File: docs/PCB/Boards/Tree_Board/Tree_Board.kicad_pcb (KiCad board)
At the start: 2 copper layers, 160 x 158 mm, 116 parts, among them Q1 AO3418, Q2 AO3418, SW1 Tact Switch 6x6mm / 13mm, U3 ATtiny85-20S

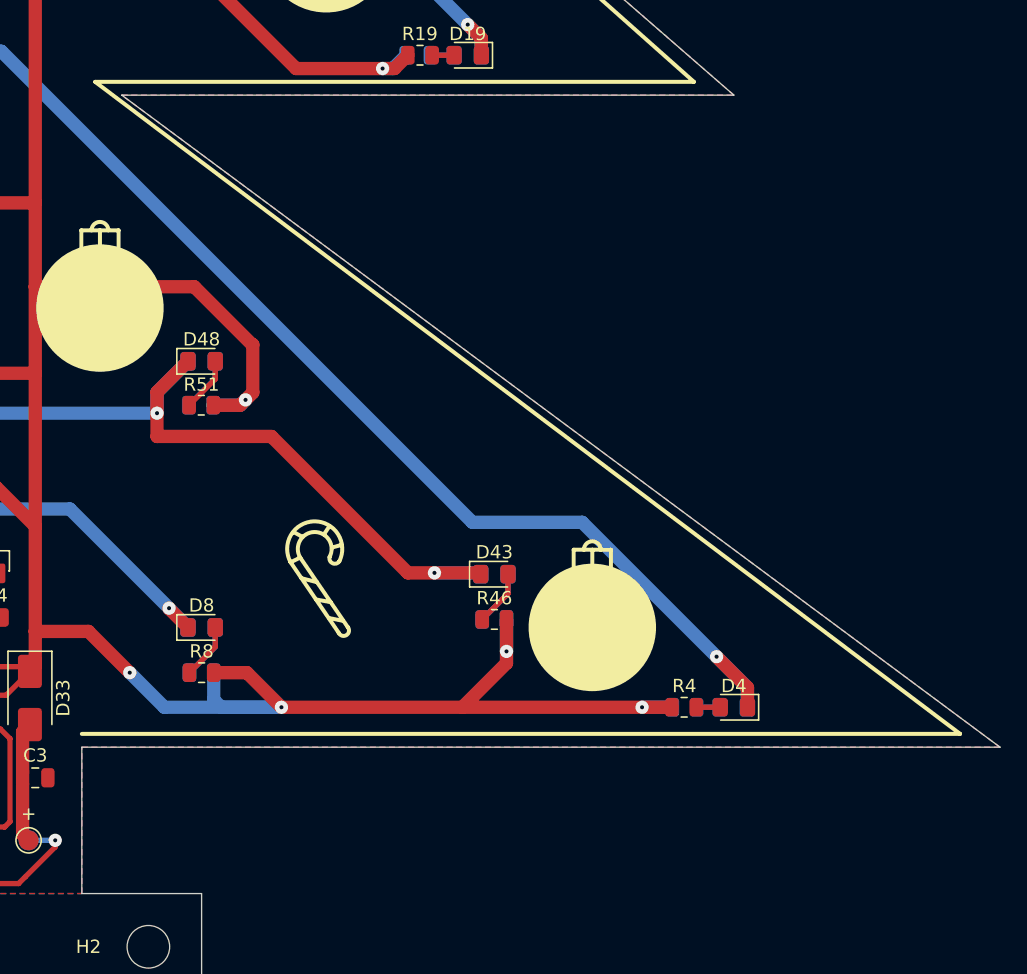
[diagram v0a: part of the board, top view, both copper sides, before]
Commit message: Boards modified.
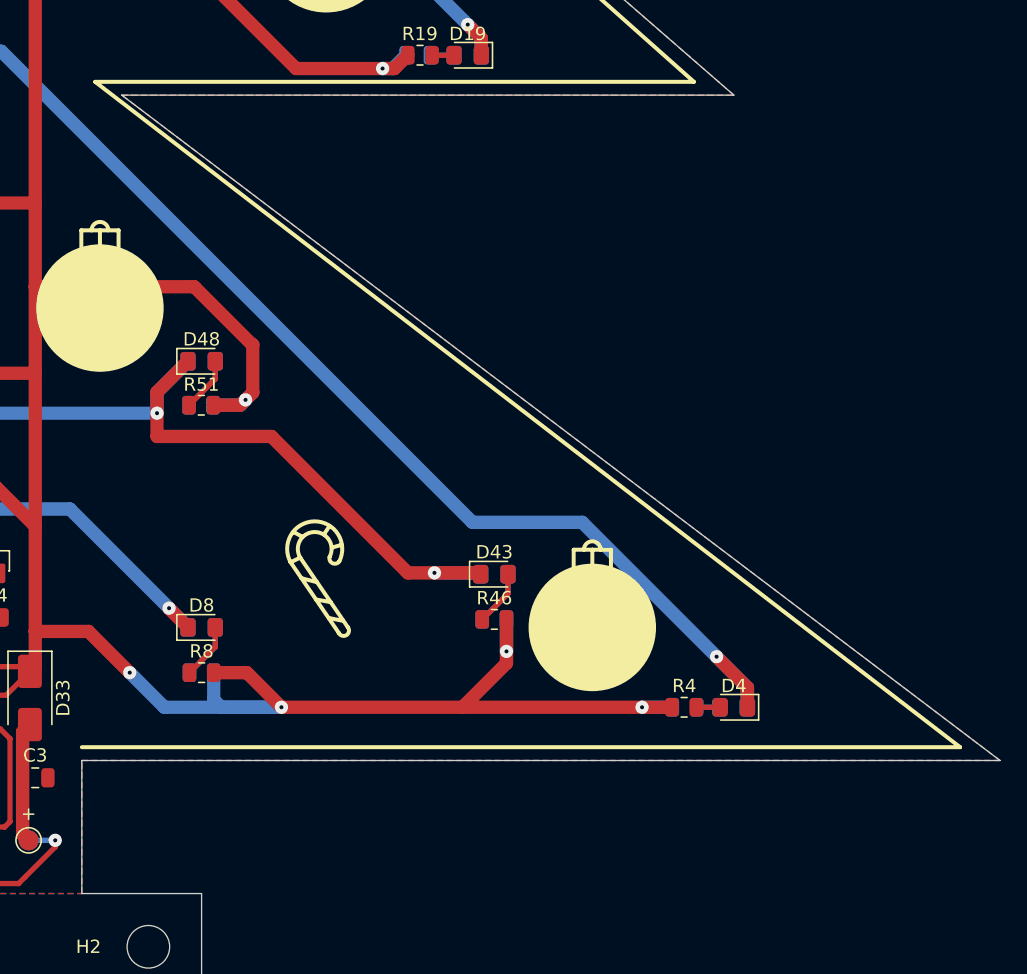
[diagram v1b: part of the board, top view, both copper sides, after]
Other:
- outline, holes or cut-outs redrawn
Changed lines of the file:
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@@
 	(title_block
 		(title "Tree_Board")
-		(date "2025-11-16")
-		(rev "1.0")
+		(date "2025-12-07")
+		(rev "1.1")
 		(company "PKl")
+		(comment 1 "Poprawiony wygląd drzewa.")
 	)
 	(layers
@@
 	)
 	(gr_line
-		(start 197 158)
-		(end 131 158)
+		(start 197 159)
+		(end 131 159)
 		(stroke
 			(width 0.3)
@@
 	(gr_line
 		(start 132 109)
-		(end 197 158)
+		(end 197 159)
 		(stroke
 			(width 0.3)
@@
 	(gr_line
 		(start 132 109)
-		(end 197 158)
+		(end 197 159)
 		(stroke
 			(width 0.3)
@@
 	)
 	(gr_line
-		(start 131 158)
-		(end 197 158)
+		(start 131 159)
+		(end 197 159)
 		(stroke
 			(width 0.3)
@@
 	)
 	(gr_line
-		(start 200 159)
-		(end 131 159)
-		(stroke
-			(width 0.05)
-			(type default)
-		)
-		(layer "Edge.Cuts")
-	)
-	(gr_line
 		(start 131 40)
 		(end 160 70)
@@
 	)
 	(gr_line
-		(start 134 110)
-		(end 200 159)
-		(stroke
-			(width 0.05)
-			(type default)
-		)
-		(layer "Edge.Cuts")
-	)
-	(gr_line
 		(start 40 160)
 		(end 109 160)
@@
 	(gr_line
 		(start 131 170)
-		(end 131 159)
+		(end 131 160)
+		(stroke
+			(width 0.05)
+			(type default)
+		)
+		(layer "Edge.Cuts")
+	)
+	(gr_line
+		(start 200 160)
+		(end 134 110)
 		(stroke
 			(width 0.05)
@@
 	)
 	(gr_line
+		(start 131 160)
+		(end 200 160)
+		(stroke
+			(width 0.05)
+			(type default)
+		)
+		(layer "Edge.Cuts")
+	)
+	(gr_line
 		(start 180 110)
 		(end 134 110)
@@
 			(pts
 				(xy 120 20) (xy 100 40) (xy 109 40) (xy 80 70) (xy 106 70) (xy 60 110) (xy 106 110) (xy 40 160)
-				(xy 109 160) (xy 109 170) (xy 131 170) (xy 131 159) (xy 200 159) (xy 134 110) (xy 180 110) (xy 134 70)
+				(xy 109 160) (xy 109 170) (xy 131 170) (xy 131 160) (xy 200 160) (xy 134 110) (xy 180 110) (xy 134 70)
 				(xy 160 70) (xy 131 40) (xy 140 40)
 			)
